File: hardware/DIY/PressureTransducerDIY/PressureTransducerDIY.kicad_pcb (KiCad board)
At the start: 2 copper layers, 66 x 48.3 mm, 13 parts, among them J1 JST_Power_Connector_Female, J2 PinHeader_Female_MS5803, J3 PinHeader_Female_Serial, U1 ATmega328P-PU, U2 MCP1700-3002E_TO92

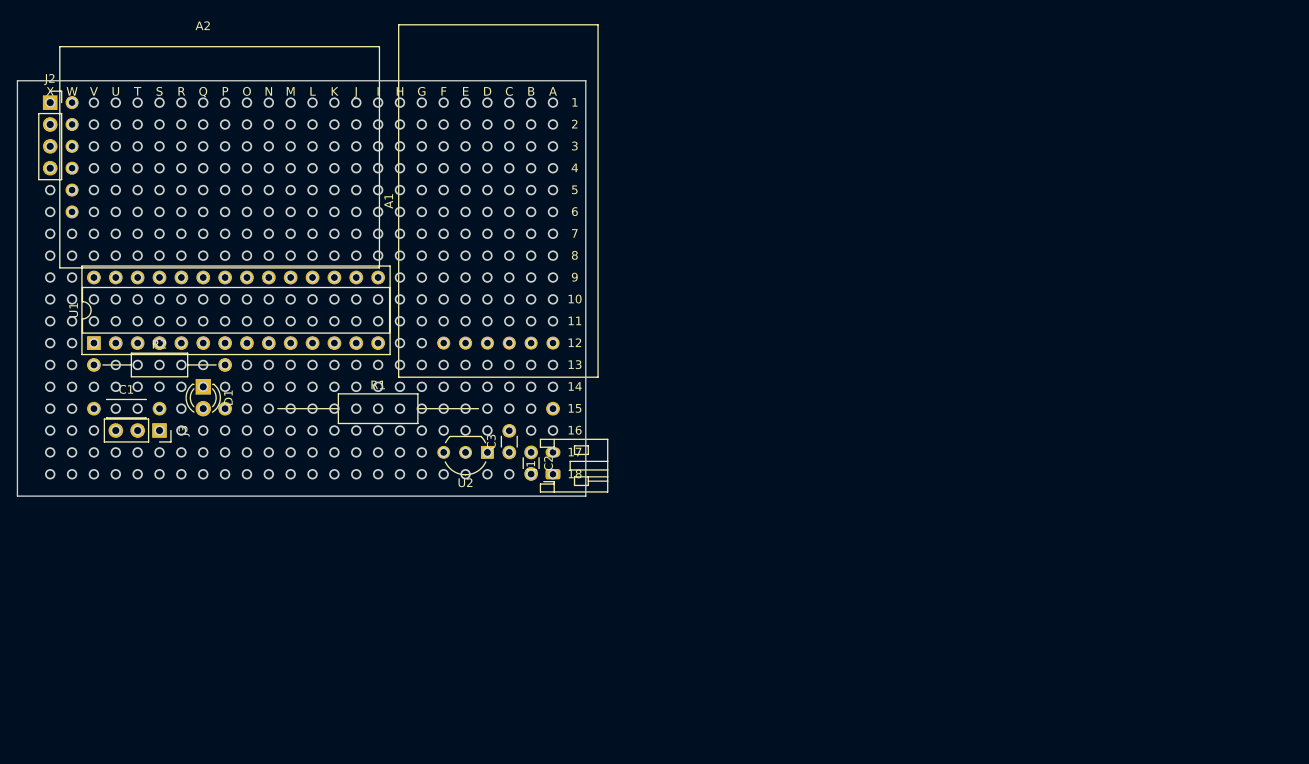
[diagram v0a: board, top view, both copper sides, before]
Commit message: Restart for new set of assembly photos
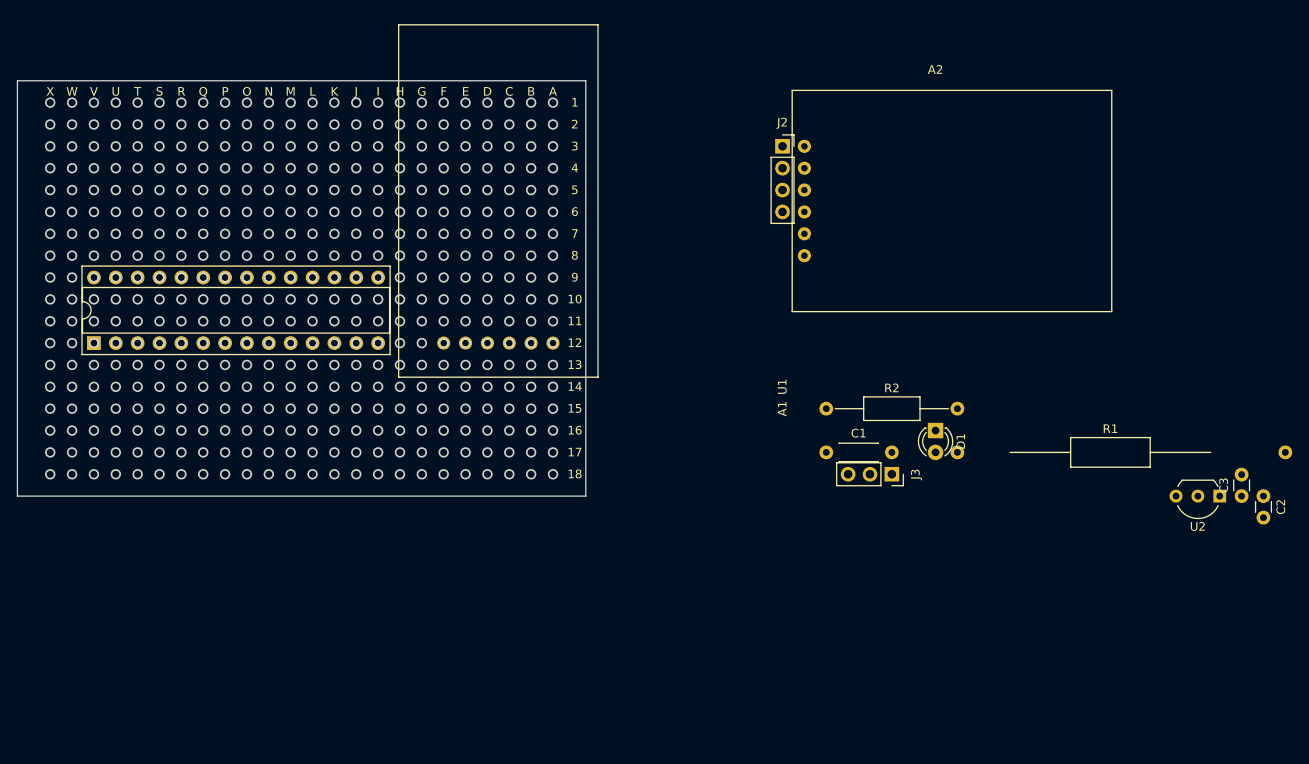
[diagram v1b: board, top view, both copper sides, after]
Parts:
- removed J1: JST_Power_Connector_Female, Connector_JST:JST_PH_S2B-PH-K_1x02_P2.00mm_Horizontal
- moved A2 85.2 mm to (245.1, 102.9)
- moved C1 85.2 mm to (233.7, 132.1)
- moved C3 85.2 mm to (280.7, 137.2)
- moved D1 85.2 mm to (245.1, 129.5)
- moved J2 85.2 mm to (227.3, 96.5)
- moved J3 85.2 mm to (240.0, 134.6)
- moved R1 85.2 mm to (252.7, 132.1)
- moved R2 85.2 mm to (232.4, 127.0)
- moved U2 85.2 mm to (278.1, 137.2)
- moved C2 85.2 mm to (283.2, 137.2)

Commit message: Finished new assembly photos
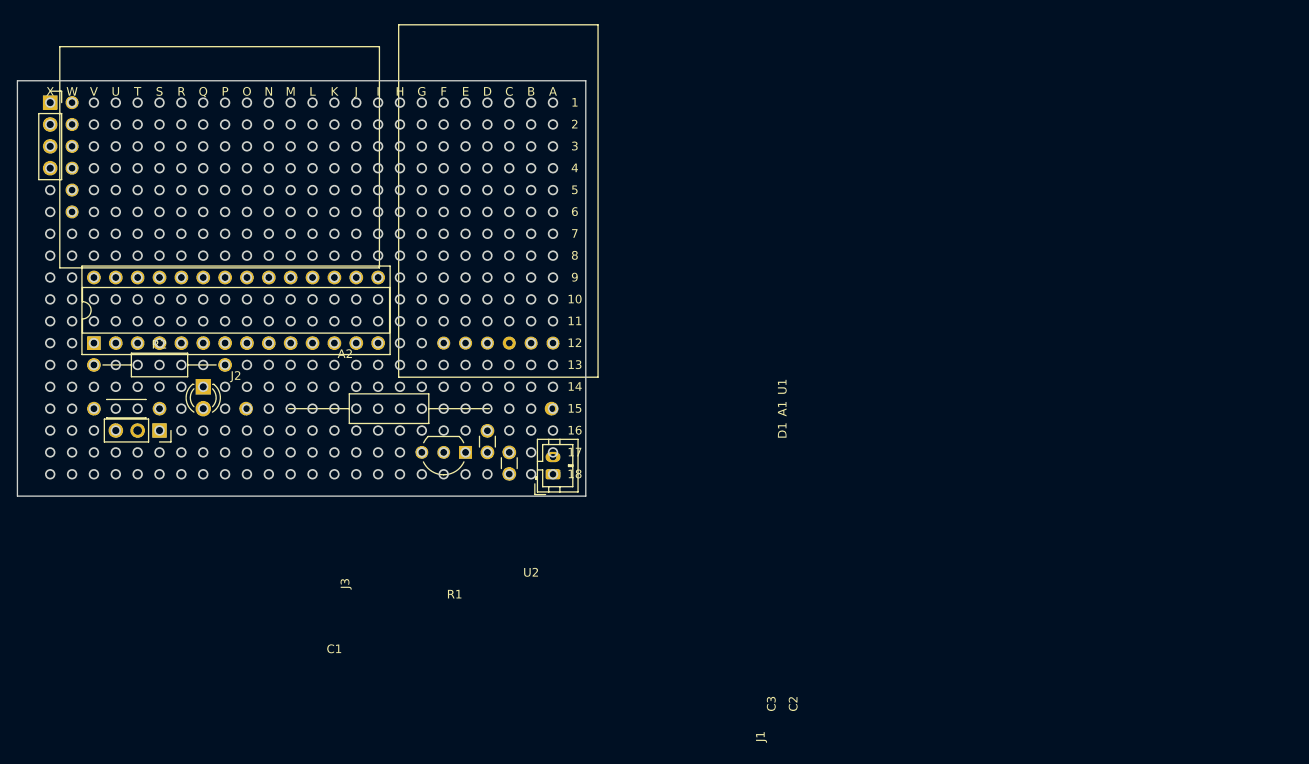
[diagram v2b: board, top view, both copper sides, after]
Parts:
- added J1: JST_Power_Connector_Female, Connector_JST:JST_PH_B2B-PH-K_1x02_P2.00mm_Vertical, F.Cu at (200.7, 134.6)
- moved C3 87.8 mm to (193.0, 132.1)
- moved U2 87.8 mm to (190.5, 132.1)
- moved C2 87.8 mm to (195.6, 132.1)
- moved A2 85.2 mm to (160.0, 97.8)
- moved C1 85.2 mm to (148.6, 127.0)
- moved D1 85.2 mm to (160.0, 124.5)
- moved J2 85.2 mm to (142.2, 91.4)
- moved J3 85.2 mm to (154.9, 129.5)
- moved R2 85.2 mm to (147.3, 121.9)
- moved R1 84.0 mm to (168.9, 127.0)
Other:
- outline, holes or cut-outs redrawn
